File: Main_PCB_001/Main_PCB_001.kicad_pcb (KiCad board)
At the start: 4 copper layers, 55 x 15 mm, 65 parts, among them IC1 FDN8601, IC2 FDN8601, IC3 TPS40211QDGQRQ1, IC4 PAM2863ECR, IC5 FDN8601, IC6 ZXTR2105FQ-7, U1 ATtiny25-20S, U2 Mounting_Hole_M2, U3 Mounting_Hole_M2, U4 Mounting_Hole_M2, U5 Mounting_Hole_M2

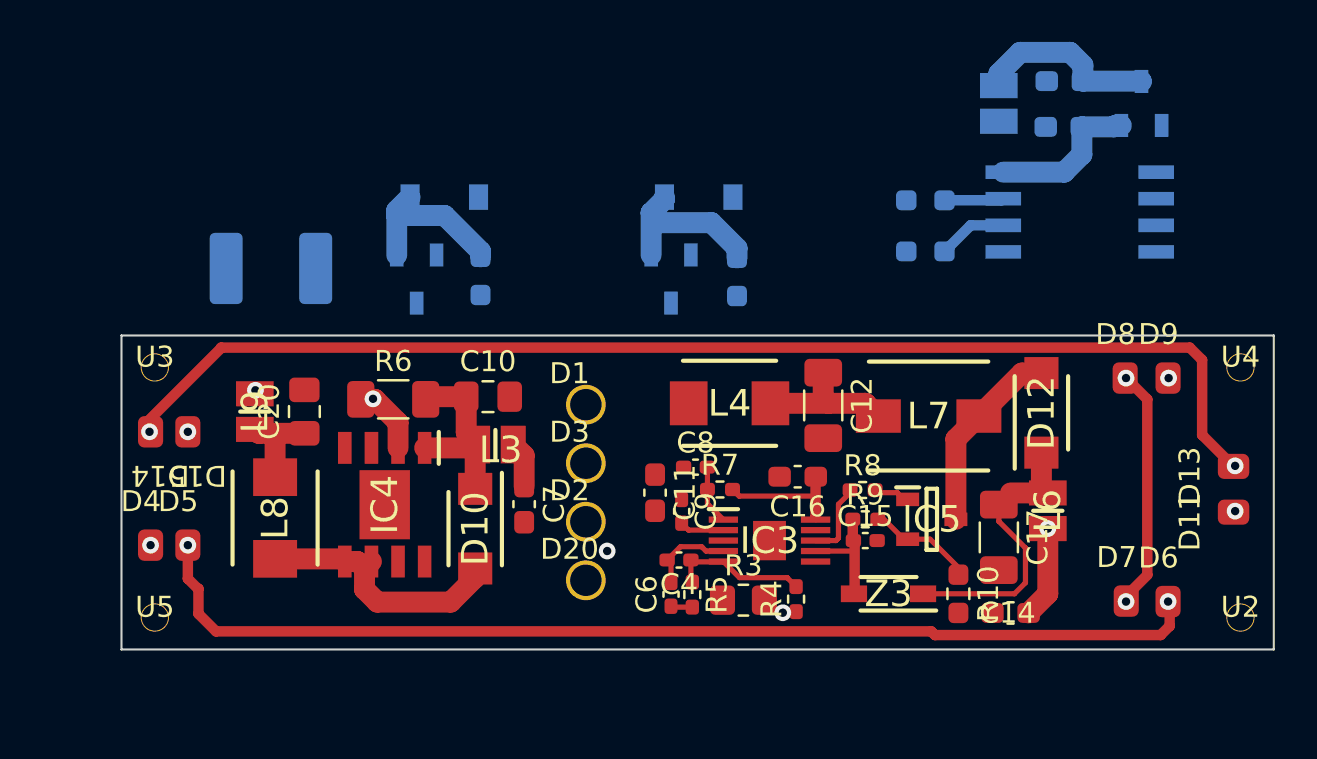
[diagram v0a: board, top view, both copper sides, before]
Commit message: PCB+Solidworks
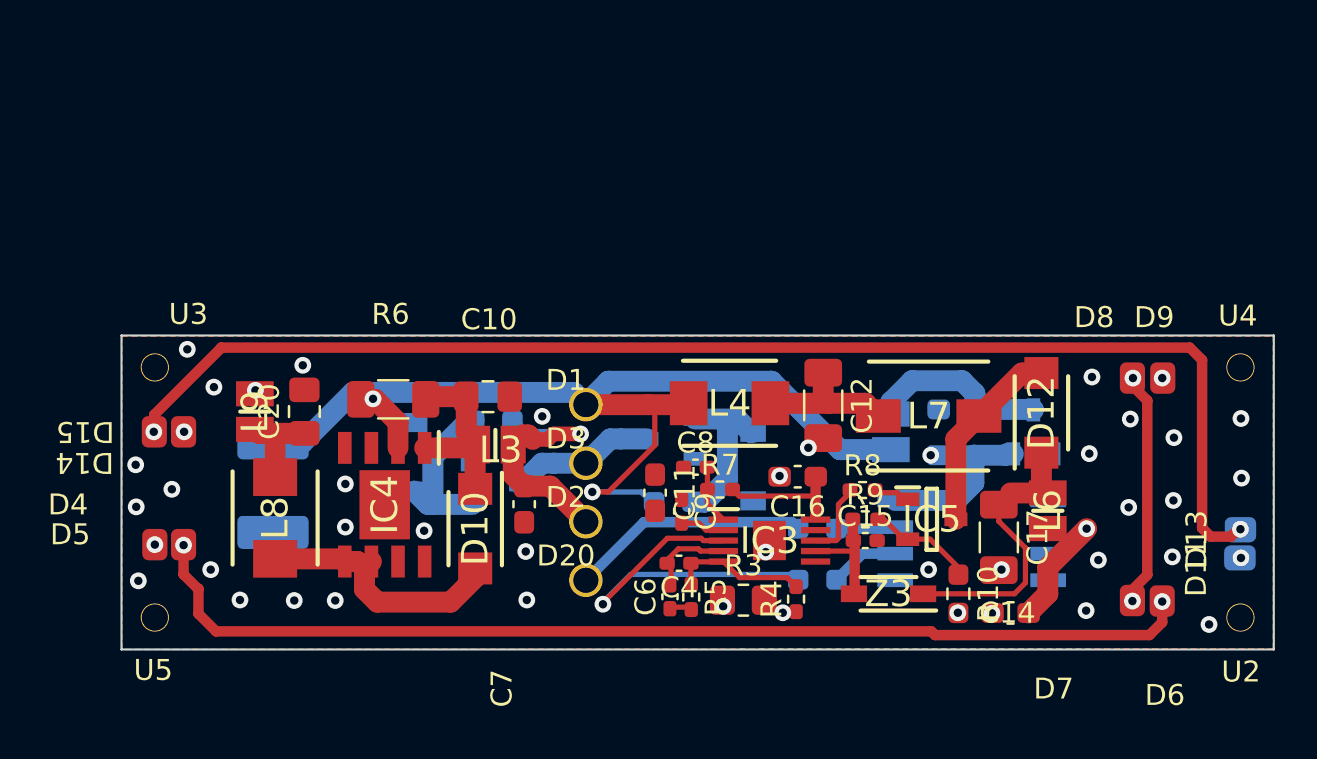
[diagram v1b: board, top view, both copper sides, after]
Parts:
- D1, D2, D20, D3: footprint libraries:WireHole_1p5 -> libraries:WireHole_1p2
- moved C22 16.5 mm to (139.8, 104.8)
- moved U1 16.5 mm to (140.6, 108.8)
- moved L10 16.5 mm to (136.7, 103.7)
- moved C23 16.5 mm to (139.9, 102.6)
- moved IC6 16.5 mm to (143.5, 103.7)
- moved R11 16.5 mm to (133.2, 110.7)
- moved R12 16.5 mm to (133.2, 108.3)
- moved Z1 13.1 mm to (130.2, 105.3), turned to -90 degrees
- moved Z2 12.5 mm to (114.0, 104.9), turned to 90 degrees
- moved R1 11.2 mm to (126.3, 107.0), turned to 0 degrees
- moved IC2 10.5 mm to (117.9, 106.2), turned to 0 degrees
- moved C21 10.5 mm to (107.2, 106.3), turned to -90 degrees
- moved IC1 7.63 mm to (126.2, 104.0), turned to 180 degrees
- moved R2 6.94 mm to (117.8, 103.1), turned to 180 degrees
- moved D13 3.04 mm to (153.4, 108.3)
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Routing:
- net Net-(C11-Pad1): track 0.00 -> 46.7 mm, vias 0 -> 1
- net Net-(IC3-Pad3): track 0.00 -> 17.2 mm
- net Net-(D20-Pad1): track 0.00 -> 11.4 mm
- net Net-(C7-Pad1): track 2.20 -> 13.0 mm, vias 0 -> 1
- net Net-(D3-Pad1): track 0.00 -> 6.93 mm
- net Net-(D13-Pad1): track 58.3 -> 63.0 mm
- net Net-(D11-Pad1): track 54.8 -> 57.0 mm
- net Net-(C14-Pad1): track 16.7 -> 15.5 mm
- net GND: vias 0 -> 38
- added copper zone on B.Cu, net GND
- added copper zone on F.Cu, net GND
- added copper zone on In1.Cu, net GND
- added copper zone on In2.Cu, net GND
